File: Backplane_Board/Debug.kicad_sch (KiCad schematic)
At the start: 11 parts, among them J44 Micro_SD_Card_Det2

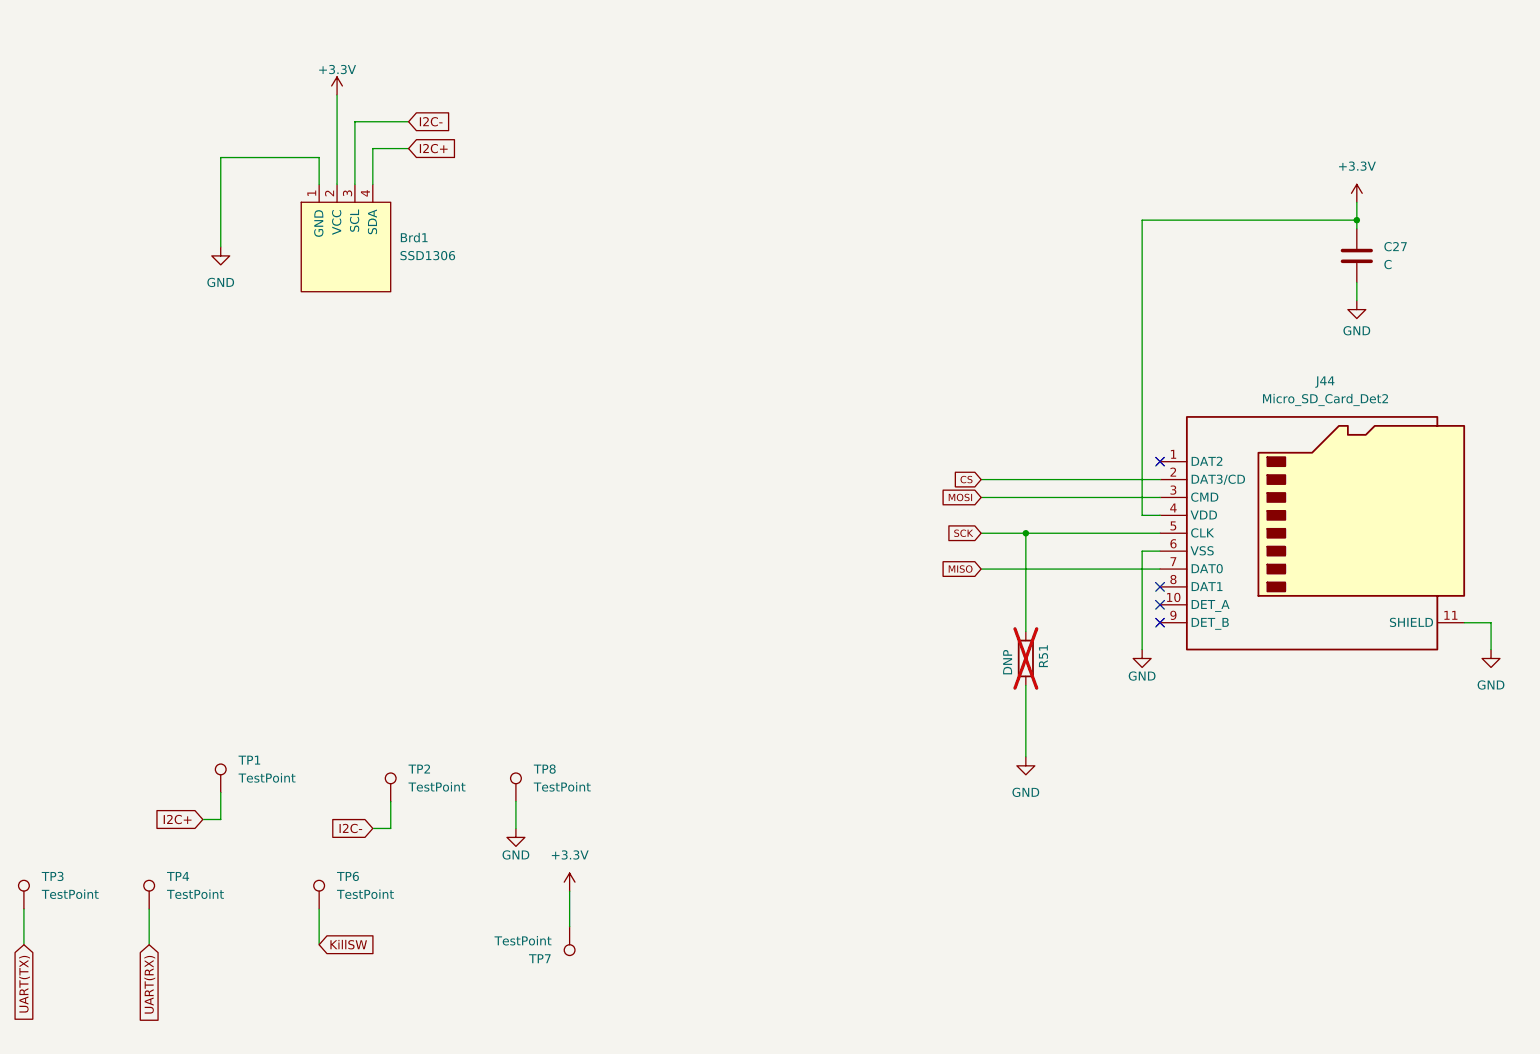
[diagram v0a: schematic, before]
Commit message: add anotations
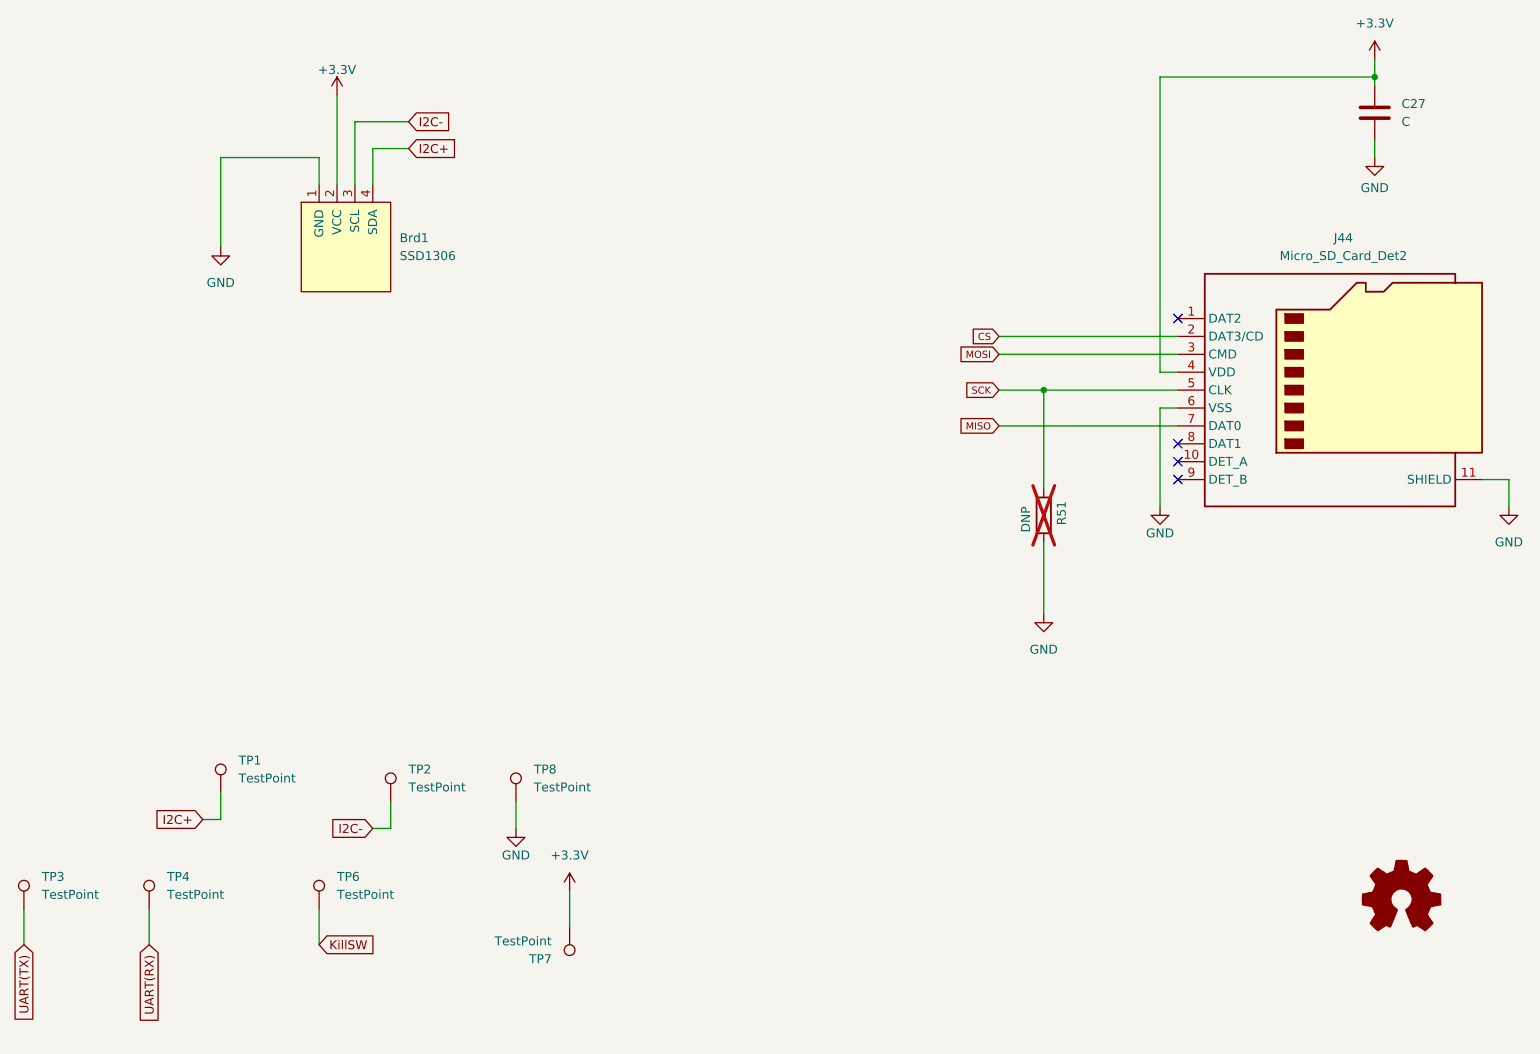
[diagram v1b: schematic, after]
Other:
- moved on the sheet: C27, J44, R51
